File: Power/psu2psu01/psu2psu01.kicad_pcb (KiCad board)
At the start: 2 copper layers, 142 x 78 mm, 132 parts, among them J1 CONN01PIN, J2 CONN01PIN, J3 CONN01PIN, J4 CONN01PIN, J5 CONN01PIN, J6 CONN01PIN, T1 HM1243, T2 YC13006, T3 HB13006, U1 DM311, U2 TL431LP, U3 817, U4 TL494IDR

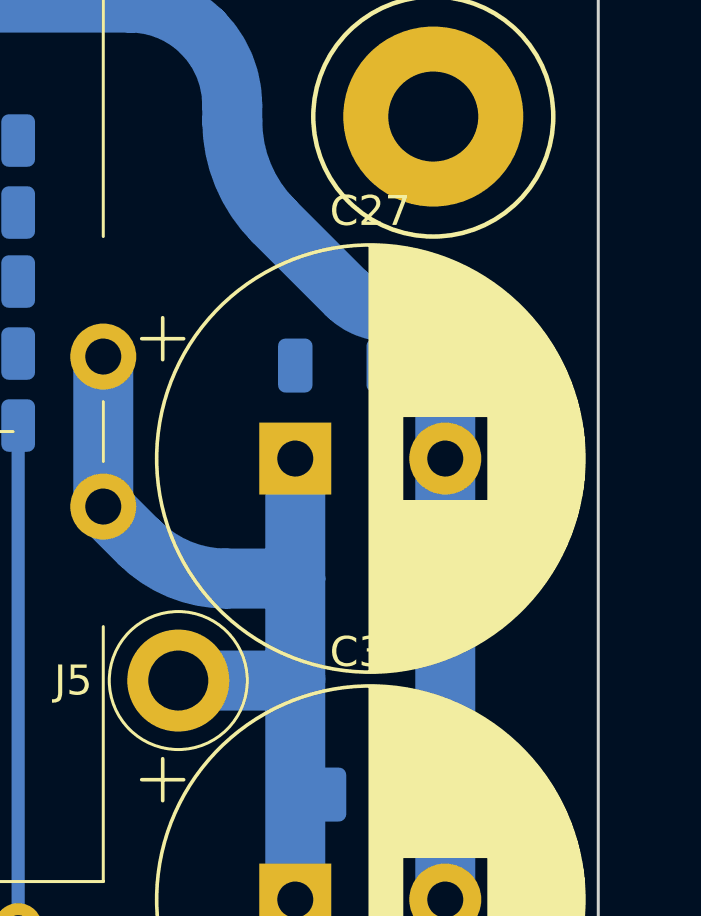
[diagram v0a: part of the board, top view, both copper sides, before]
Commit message: up
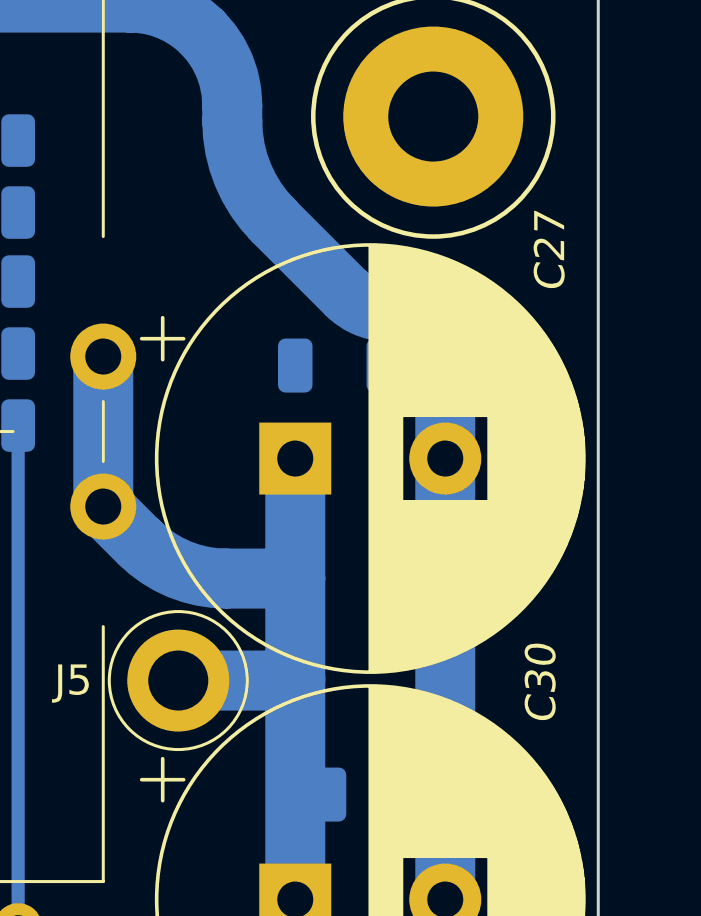
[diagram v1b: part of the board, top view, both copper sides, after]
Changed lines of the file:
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@@
     (property "ki_description" "Конденсатор полярный")
     (attr through_hole)
-    (fp_text reference "C30" (at 2.5 -8.25) (layer "F.SilkS")
-        (effects (font (size 1 1) (thickness 0.15)))
+    (fp_text reference "C30" (at 8.2 -7.2 90) (layer "F.SilkS")
+        (effects (font (size 1 1) (thickness 0.15) italic))
     )
     (fp_text value "470x63" (at 2.5 8.25) (layer "F.Fab")
@@
     (property "ki_description" "Конденсатор полярный")
     (attr through_hole)
-    (fp_text reference "C27" (at 2.5 -8.25) (layer "F.SilkS")
-        (effects (font (size 1 1) (thickness 0.15)))
+    (fp_text reference "C27" (at 8.5 -6.9 90) (layer "F.SilkS")
+        (effects (font (size 1 1) (thickness 0.15) italic))
     )
     (fp_text value "470x63" (at 2.5 8.25) (layer "F.Fab")
